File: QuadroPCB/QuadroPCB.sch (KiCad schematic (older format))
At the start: 23 parts, among them IC1 AT24CS02-SSHM, P1 MPU9150, P10 AKKU, P2 stm32discovery_left, P3 stm32discovery_right, P4 rc_signal, P5 Motor3, P6 Motor4, P7 BMP180, P8 Motor1, P9 Motor2, Q1 Q_NMOS_GSD, U1 LM2576S-5

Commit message: dei mudder commitet
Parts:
- P10: footprint Wire_Connections_Bridges:WireConnection_1-2mmDrill -> Connect:PINHEAD1-2
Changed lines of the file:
@@
 F 0 "P10" H 1000 1750 50  0000 C CNN
 F 1 "AKKU" V 1100 1600 50  0000 C CNN
-F 2 "Wire_Connections_Bridges:WireConnection_1-2mmDrill" H 1000 1600 60  0001 C CNN
+F 2 "Connect:PINHEAD1-2" H 1000 1600 60  0001 C CNN
 F 3 "" H 1000 1600 60  0000 C CNN
 	1    1000 1600

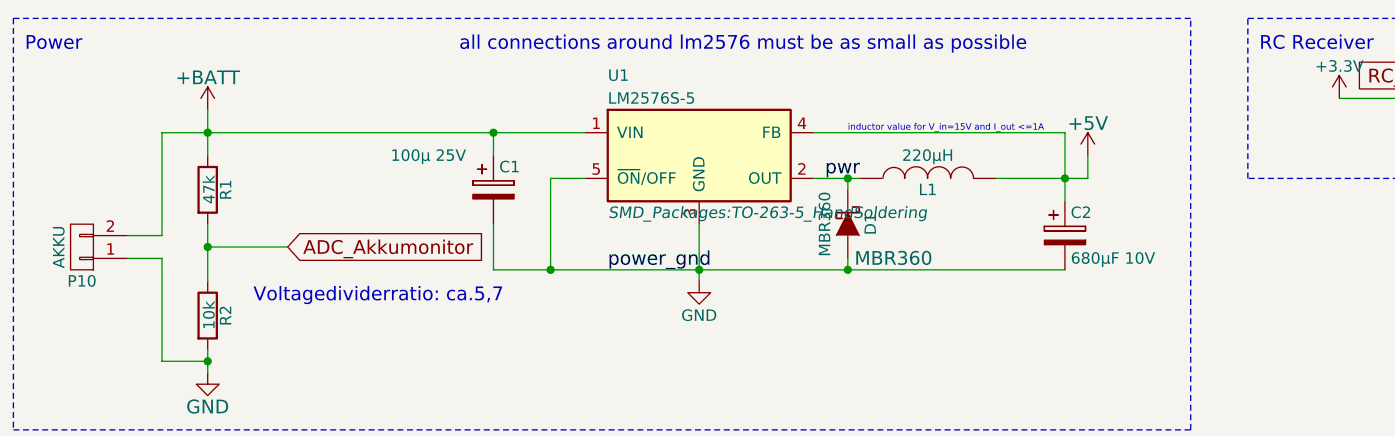
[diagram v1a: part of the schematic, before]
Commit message: neuer step down
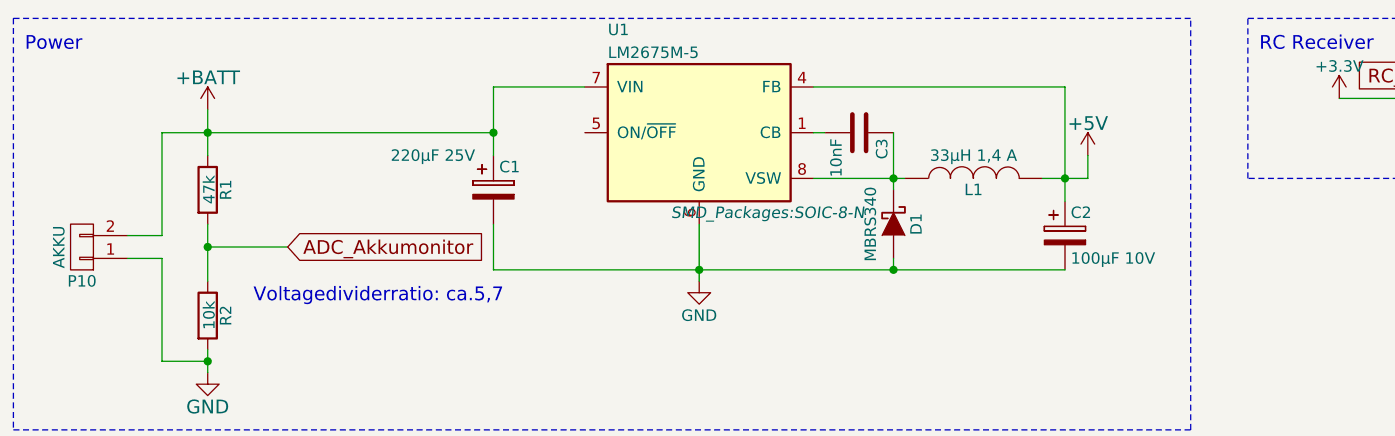
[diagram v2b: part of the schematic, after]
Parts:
- removed U1: LM2576S-5, SMD_Packages:TO-263-5_HandSoldering, symbol LM2576S-5
- added C3: 10nF, Capacitors_SMD:C_0805_HandSoldering, symbol C
- added U1: LM2675M-5, SMD_Packages:SOIC-8-N, symbol LM2675M-5
- C1: value 100µ 25V -> 220µF 25V; footprint Capacitors_SMD:c_elec_6.3x7.7 -> Capacitors_SMD:c_elec_8x10.5
- C2: value 680µF 10V -> 100µF 10V; footprint Capacitors_SMD:c_elec_8x10 -> Capacitors_SMD:c_elec_8x6.7
- D1: value MBR360 -> MBRS340; footprint Diodes_SMD:Diode-DO-214BA -> Diodes_SMD:Diode-DO-214AB_Handsoldering; type MBR360 -> (none)
- L1: value 220µH -> 33µH 1,4 A; footprint Choke_SMD:Choke_SMD_PISR_Handsoldering_FASTRON -> Choke_SMD:Choke_SMD_PISN_Handsoldering_FASTRON
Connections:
- net +5V: now also U1.4 (FB)
- net +BATT: now also U1.7 (VIN)
- net GND: now also U1.6 (GND)
- net pwr: no longer names the net of D1.1 (K), L1.1
- net pwr: now also C3.1, U1.8 (VSW)
- new net: C3.2, U1.1 (CB)
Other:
- note removed: "all connections around lm2576 must be as small as possible"
- note removed: "inductor value for V_in=15V and I_out <=1A"
- moved on the sheet: D1, L1
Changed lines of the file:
@@
 $EndComp
 $Comp
-L GND #PWR01
+L GND #PWR5
 U 1 1 553FEFAB
 P 1550 2150
-F 0 "#PWR01" H 1550 1900 60  0001 C CNN
+F 0 "#PWR5" H 1550 1900 60  0001 C CNN
 F 1 "GND" H 1550 2000 60  0000 C CNN
 F 2 "" H 1550 2150 60  0000 C CNN
@@
 $EndComp
 $Comp
-L +BATT #PWR02
+L +BATT #PWR4
 U 1 1 553FEFC1
 P 1550 1000
-F 0 "#PWR02" H 1550 850 60  0001 C CNN
+F 0 "#PWR4" H 1550 850 60  0001 C CNN
 F 1 "+BATT" H 1550 1140 60  0000 C CNN
 F 2 "" H 1550 1000 60  0000 C CNN
@@
 	1900 1600 1550 1600
 Connection ~ 1550 1600
-Wire Wire Line
-	1350 1100 3200 1100
 Connection ~ 1550 1100
 $Comp
-L +5V #PWR03
+L +5V #PWR11
 U 1 1 553FF02F
 P 5400 1200
-F 0 "#PWR03" H 5400 1050 60  0001 C CNN
+F 0 "#PWR11" H 5400 1050 60  0001 C CNN
 F 1 "+5V" H 5400 1340 60  0000 C CNN
 F 2 "" H 5400 1200 60  0000 C CNN
@@
 $EndComp
 $Comp
-L GND #PWR04
+L GND #PWR15
 U 1 1 553FF2AD
 P 8700 1150
-F 0 "#PWR04" H 8700 900 60  0001 C CNN
+F 0 "#PWR15" H 8700 900 60  0001 C CNN
 F 1 "GND" H 8700 1000 60  0000 C CNN
 F 2 "" H 8700 1150 60  0000 C CNN
@@
 $EndComp
 $Comp
-L +3V3 #PWR05
+L +3V3 #PWR14
 U 1 1 553FF331
 P 8500 1000
-F 0 "#PWR05" H 8500 850 60  0001 C CNN
+F 0 "#PWR14" H 8500 850 60  0001 C CNN
 F 1 "+3V3" H 8500 1140 60  0000 C CNN
 F 2 "" H 8500 1000 60  0000 C CNN
@@
 Voltagedividerratio: ca.5,7\n
 $Comp
-L LM2576S-5 U1
-U 1 1 5541EC13
-P 3700 1200
-F 0 "U1" H 3300 1550 50  0000 L CNN
-F 1 "LM2576S-5" H 3300 1450 50  0000 L CNN
-F 2 "SMD_Packages:TO-263-5_HandSoldering" H 4000 950 50  0000 C CIN
-F 3 "" H 3700 1200 50  0000 C CNN
-	1    3700 1200
-	1    0    0    -1
-$EndComp
-$Comp
-L GND #PWR06
+L GND #PWR10
 U 1 1 5541ECA6
 P 3700 1750
-F 0 "#PWR06" H 3700 1500 50  0001 C CNN
+F 0 "#PWR10" H 3700 1500 50  0001 C CNN
 F 1 "GND" H 3700 1600 50  0000 C CNN
 F 2 "" H 3700 1750 60  0000 C CNN
@@
 $EndComp
 Wire Wire Line
-	3700 1500 3700 1750
-Wire Wire Line
-	3200 1300 3050 1300
-Wire Wire Line
-	3050 1300 3050 1700
-Wire Wire Line
 	2800 1700 5300 1700
 Connection ~ 3700 1700
@@
 L INDUCTOR L1
 U 1 1 5541EE99
-P 4700 1300
-F 0 "L1" V 4650 1300 50  0000 C CNN
-F 1 "220µH" V 4800 1300 50  0000 C CNN
-F 2 "Choke_SMD:Choke_SMD_PISR_Handsoldering_FASTRON" H 4700 1300 60  0001 C CNN
-F 3 "" H 4700 1300 60  0000 C CNN
-	1    4700 1300
+P 4900 1300
+F 0 "L1" V 4850 1300 50  0000 C CNN
+F 1 "33µH 1,4 A" V 5000 1300 50  0000 C CNN
+F 2 "Choke_SMD:Choke_SMD_PISN_Handsoldering_FASTRON" H 4900 1300 60  0001 C CNN
+F 3 "" H 4900 1300 60  0000 C CNN
+	1    4900 1300
 	0    -1   -1   0
 $EndComp
@@
 P 5300 1550
 F 0 "C2" H 5325 1650 50  0000 L CNN
-F 1 "680µF 10V" H 5325 1450 50  0000 L CNN
-F 2 "Capacitors_SMD:c_elec_8x10" H 5338 1400 30  0001 C CNN
+F 1 "100µF 10V" H 5325 1450 50  0000 L CNN
+F 2 "Capacitors_SMD:c_elec_8x6.7" H 5338 1400 30  0001 C CNN
 F 3 "" H 5300 1550 60  0000 C CNN
 	1    5300 1550
@@
 P 2800 1350
 F 0 "C1" H 2825 1450 50  0000 L CNN
-F 1 "100µ 25V" H 2350 1500 50  0000 L CNN
-F 2 "Capacitors_SMD:c_elec_6.3x7.7" H 2838 1200 30  0001 C CNN
+F 1 "220µF 25V" H 2350 1500 50  0000 L CNN
+F 2 "Capacitors_SMD:c_elec_8x10.5" H 2838 1200 30  0001 C CNN
 F 3 "" H 2800 1350 60  0000 C CNN
 	1    2800 1350
@@
 Wire Wire Line
 	2800 1500 2800 1700
-Connection ~ 3050 1700
-Wire Wire Line
-	2800 1200 2800 1100
+Wire Wire Line
+	2800 900  2800 1200
 Connection ~ 2800 1100
 Wire Wire Line
-	4200 1300 4400 1300
-Wire Wire Line
-	5000 1300 5400 1300
+	4200 1300 4600 1300
+Wire Wire Line
+	5200 1300 5400 1300
 Connection ~ 5300 1300
 $Comp
 L D_Schottky D1
 U 1 1 5541F140
-P 4350 1500
-F 0 "D1" H 4350 1600 50  0000 C CNN
-F 1 "MBR360" H 4350 1400 50  0000 C CNN
-F 2 "Diodes_SMD:Diode-DO-214BA" H 4350 1500 60  0001 C CNN
-F 3 "" H 4350 1500 60  0000 C CNN
-F 4 "MBR360" V 4500 1700 60  0000 C CNN "type"
-	1    4350 1500
+P 4550 1500
+F 0 "D1" H 4550 1600 50  0000 C CNN
+F 1 "MBRS340" H 4550 1400 50  0000 C CNN
+F 2 "Diodes_SMD:Diode-DO-214AB_Handsoldering" H 4550 1500 60  0001 C CNN
+F 3 "" H 4550 1500 60  0000 C CNN
+	1    4550 1500
 	0    1    1    0
 $EndComp
 Wire Wire Line
-	4350 1350 4350 1300
-Connection ~ 4350 1300
-Wire Wire Line
-	4350 1650 4350 1700
-Connection ~ 4350 1700
-Wire Wire Line
-	5300 1100 5300 1400
-Text Notes 2650 750  0    60   ~ 0
-all connections around lm2576 must be as small as possible
-Text Notes 4350 1100 0    28   ~ 0
-inductor value for V_in=15V and I_out <=1A
-Wire Wire Line
-	5300 1100 4200 1100
+	4550 1100 4550 1350
+Connection ~ 4550 1300
+Wire Wire Line
+	4550 1650 4550 1700
+Connection ~ 4550 1700
 $Comp
 L R R4
@@
 $EndComp
 $Comp
-L +5V #PWR07
+L +5V #PWR22
 U 1 1 554200B8
 P 10600 900
-F 0 "#PWR07" H 10600 750 50  0001 C CNN
+F 0 "#PWR22" H 10600 750 50  0001 C CNN
 F 1 "+5V" H 10600 1040 50  0000 C CNN
 F 2 "" H 10600 900 60  0000 C CNN
@@
 $EndComp
 $Comp
-L GND #PWR08
+L GND #PWR23
 U 1 1 55420164
 P 10600 1750
-F 0 "#PWR08" H 10600 1500 50  0001 C CNN
+F 0 "#PWR23" H 10600 1500 50  0001 C CNN
 F 1 "GND" H 10600 1600 50  0000 C CNN
 F 2 "" H 10600 1750 60  0000 C CNN
@@
 $EndComp
 $Comp
-L GND #PWR09
+L GND #PWR21
 U 1 1 55420E59
 P 10400 2600
-F 0 "#PWR09" H 10400 2350 60  0001 C CNN
+F 0 "#PWR21" H 10400 2350 60  0001 C CNN
 F 1 "GND" H 10400 2450 60  0000 C CNN
 F 2 "" H 10400 2600 60  0000 C CNN
@@
 $EndComp
 $Comp
-L +3V3 #PWR010
+L +3V3 #PWR18
 U 1 1 5542137E
 P 10000 3350
-F 0 "#PWR010" H 10000 3200 60  0001 C CNN
+F 0 "#PWR18" H 10000 3200 60  0001 C CNN
 F 1 "+3V3" H 10000 3490 60  0000 C CNN
 F 2 "" H 10000 3350 60  0000 C CNN
@@
 $EndComp
 $Comp
-L GND #PWR011
+L GND #PWR19
 U 1 1 554213A3
 P 10000 4200
-F 0 "#PWR011" H 10000 3950 60  0001 C CNN
+F 0 "#PWR19" H 10000 3950 60  0001 C CNN
 F 1 "GND" H 10000 4050 60  0000 C CNN
 F 2 "" H 10000 4200 60  0000 C CNN
@@
 $EndComp
 $Comp
-L +3V3 #PWR012
+L +3V3 #PWR20
 U 1 1 55420E36
 P 10300 2300
-F 0 "#PWR012" H 10300 2150 60  0001 C CNN
+F 0 "#PWR20" H 10300 2150 60  0001 C CNN
 F 1 "+3V3" H 10300 2440 60  0000 C CNN
 F 2 "" H 10300 2300 60  0000 C CNN
@@
 	3600 2550 700  2550
 $Comp
-L +3V3 #PWR013
+L +3V3 #PWR1
 U 1 1 55422E4A
 P 1100 3300
-F 0 "#PWR013" H 1100 3150 60  0001 C CNN
+F 0 "#PWR1" H 1100 3150 60  0001 C CNN
 F 1 "+3V3" H 1100 3440 60  0000 C CNN
 F 2 "" H 1100 3300 60  0000 C CNN
@@
 $EndComp
 $Comp
-L +3V3 #PWR014
+L +3V3 #PWR6
 U 1 1 55422ECC
 P 1850 3300
-F 0 "#PWR014" H 1850 3150 60  0001 C CNN
+F 0 "#PWR6" H 1850 3150 60  0001 C CNN
 F 1 "+3V3" H 1850 3440 60  0000 C CNN
 F 2 "" H 1850 3300 60  0000 C CNN
@@
 $EndComp
 $Comp
-L GND #PWR015
+L GND #PWR2
 U 1 1 5542303C
 P 1100 3500
-F 0 "#PWR015" H 1100 3250 50  0001 C CNN
+F 0 "#PWR2" H 1100 3250 50  0001 C CNN
 F 1 "GND" H 1100 3350 50  0000 C CNN
 F 2 "" H 1100 3500 60  0000 C CNN
@@
 $EndComp
 $Comp
-L GND #PWR016
+L GND #PWR3
 U 1 1 55423070
 P 1150 6000
-F 0 "#PWR016" H 1150 5750 50  0001 C CNN
+F 0 "#PWR3" H 1150 5750 50  0001 C CNN
 F 1 "GND" H 1150 5850 50  0000 C CNN
 F 2 "" H 1150 6000 60  0000 C CNN
@@
 	1850 3400 1850 3300
 $Comp
-L +5V #PWR017
+L +5V #PWR7
 U 1 1 554236B8
 P 2400 3300
-F 0 "#PWR017" H 2400 3150 60  0001 C CNN
+F 0 "#PWR7" H 2400 3150 60  0001 C CNN
 F 1 "+5V" H 2400 3440 60  0000 C CNN
 F 2 "" H 2400 3300 60  0000 C CNN
@@
 	2400 3400 2400 3300
 $Comp
-L +5V #PWR018
+L +5V #PWR9
 U 1 1 554237F2
 P 3100 3300
-F 0 "#PWR018" H 3100 3150 60  0001 C CNN
+F 0 "#PWR9" H 3100 3150 60  0001 C CNN
 F 1 "+5V" H 3100 3440 60  0000 C CNN
 F 2 "" H 3100 3300 60  0000 C CNN
@@
 	3100 3400 3100 3300
 $Comp
-L GND #PWR019
+L GND #PWR8
 U 1 1 554239AA
 P 2450 6000
-F 0 "#PWR019" H 2450 5750 50  0001 C CNN
+F 0 "#PWR8" H 2450 5750 50  0001 C CNN
 F 1 "GND" H 2450 5850 50  0000 C CNN
 F 2 "" H 2450 6000 60  0000 C CNN
@@
 $EndComp
 $Comp
-L +3.3V #PWR020
+L +3.3V #PWR12
 U 1 1 55423C5D
 P 6500 950
-F 0 "#PWR020" H 6500 800 50  0001 C CNN
+F 0 "#PWR12" H 6500 800 50  0001 C CNN
 F 1 "+3.3V" H 6500 1090 50  0000 C CNN
 F 2 "" H 6500 950 60  0000 C CNN
@@
 $EndComp
 $Comp
-L GND #PWR021
+L GND #PWR13
 U 1 1 55423C83
 P 7100 1100
-F 0 "#PWR021" H 7100 850 50  0001 C CNN
+F 0 "#PWR13" H 7100 850 50  0001 C CNN
 F 1 "GND" H 7100 950 50  0000 C CNN
 F 2 "" H 7100 1100 60  0000 C CNN
@@
 MOTOR4
 $Comp
-L GND #PWR022
+L GND #PWR17
 U 1 1 554248D9
 P 9700 5550
-F 0 "#PWR022" H 9700 5300 50  0001 C CNN
+F 0 "#PWR17" H 9700 5300 50  0001 C CNN
 F 1 "GND" H 9700 5400 50  0000 C CNN
 F 2 "" H 9700 5550 60  0000 C CNN
@@
 $EndComp
 $Comp
-L GND #PWR023
+L GND #PWR16
 U 1 1 55424917
 P 9700 5050
-F 0 "#PWR023" H 9700 4800 50  0001 C CNN
+F 0 "#PWR16" H 9700 4800 50  0001 C CNN
 F 1 "GND" H 9700 4900 50  0000 C CNN
 F 2 "" H 9700 5050 60  0000 C CNN
@@
 $EndComp
 $Comp
-L GND #PWR024
+L GND #PWR25
 U 1 1 5542494E
 P 10600 5600
-F 0 "#PWR024" H 10600 5350 50  0001 C CNN
+F 0 "#PWR25" H 10600 5350 50  0001 C CNN
 F 1 "GND" H 10600 5450 50  0000 C CNN
 F 2 "" H 10600 5600 60  0000 C CNN
@@
 $EndComp
 $Comp
-L GND #PWR025
+L GND #PWR24
 U 1 1 5542499B
 P 10600 5050
-F 0 "#PWR025" H 10600 4800 50  0001 C CNN
+F 0 "#PWR24" H 10600 4800 50  0001 C CNN
 F 1 "GND" H 10600 4900 50  0000 C CNN
 F 2 "" H 10600 5050 60  0000 C CNN
@@
 Wire Wire Line
 	1350 1550 1350 1100
-Text Label 3300 1700 0    60   ~ 0
-power_gnd
-Text Label 4250 1300 0    60   ~ 0
-pwr
+$Comp
+L LM2675M-5 U1
+U 1 1 55461C96
+P 3700 1100
+F 0 "U1" H 3300 1550 50  0000 L CNN
+F 1 "LM2675M-5" H 3300 1450 50  0000 L CNN
+F 2 "SMD_Packages:SOIC-8-N" H 4000 750 50  0000 C CIN
+F 3 "" H 3700 1100 50  0000 C CNN
+	1    3700 1100
+	1    0    0    -1
+$EndComp
+Wire Wire Line
+	3700 1500 3700 1750
+Wire Wire Line
+	3200 900  2800 900
+Wire Wire Line
+	1350 1100 2800 1100
+$Comp
+L C C3
+U 1 1 554623AC
+P 4400 1100
+F 0 "C3" H 4425 1200 50  0000 L CNN
+F 1 "10nF" H 4425 1000 50  0000 L CNN
+F 2 "Capacitors_SMD:C_0805_HandSoldering" H 4438 950 30  0001 C CNN
+F 3 "" H 4400 1100 60  0000 C CNN
+	1    4400 1100
+	0    1    1    0
+$EndComp
+Wire Wire Line
+	4200 1100 4250 1100
+Wire Wire Line
+	4200 900  5300 900
+Wire Wire Line
+	5300 900  5300 1400
 $EndSCHEMATC
